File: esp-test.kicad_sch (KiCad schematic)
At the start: 77 parts, among them J1 AudioPlug3, J2 Micro_SD_Card_Det1, J3 USB_C_Receptacle_USB2.0_14P, J4 USB_C_Receptacle_USB2.0_14P, J5 Micro_SD_Card_Det2, SW1 Volume Up, SW2 Volume Down, SW3 Up, SW4 Down, SW5 Left, SW6 Right, SW7 SW_SPST, U1 ESP32-S3-WROOM-1, U2 AP2112K-3.3, U4 AP2112K-3.3

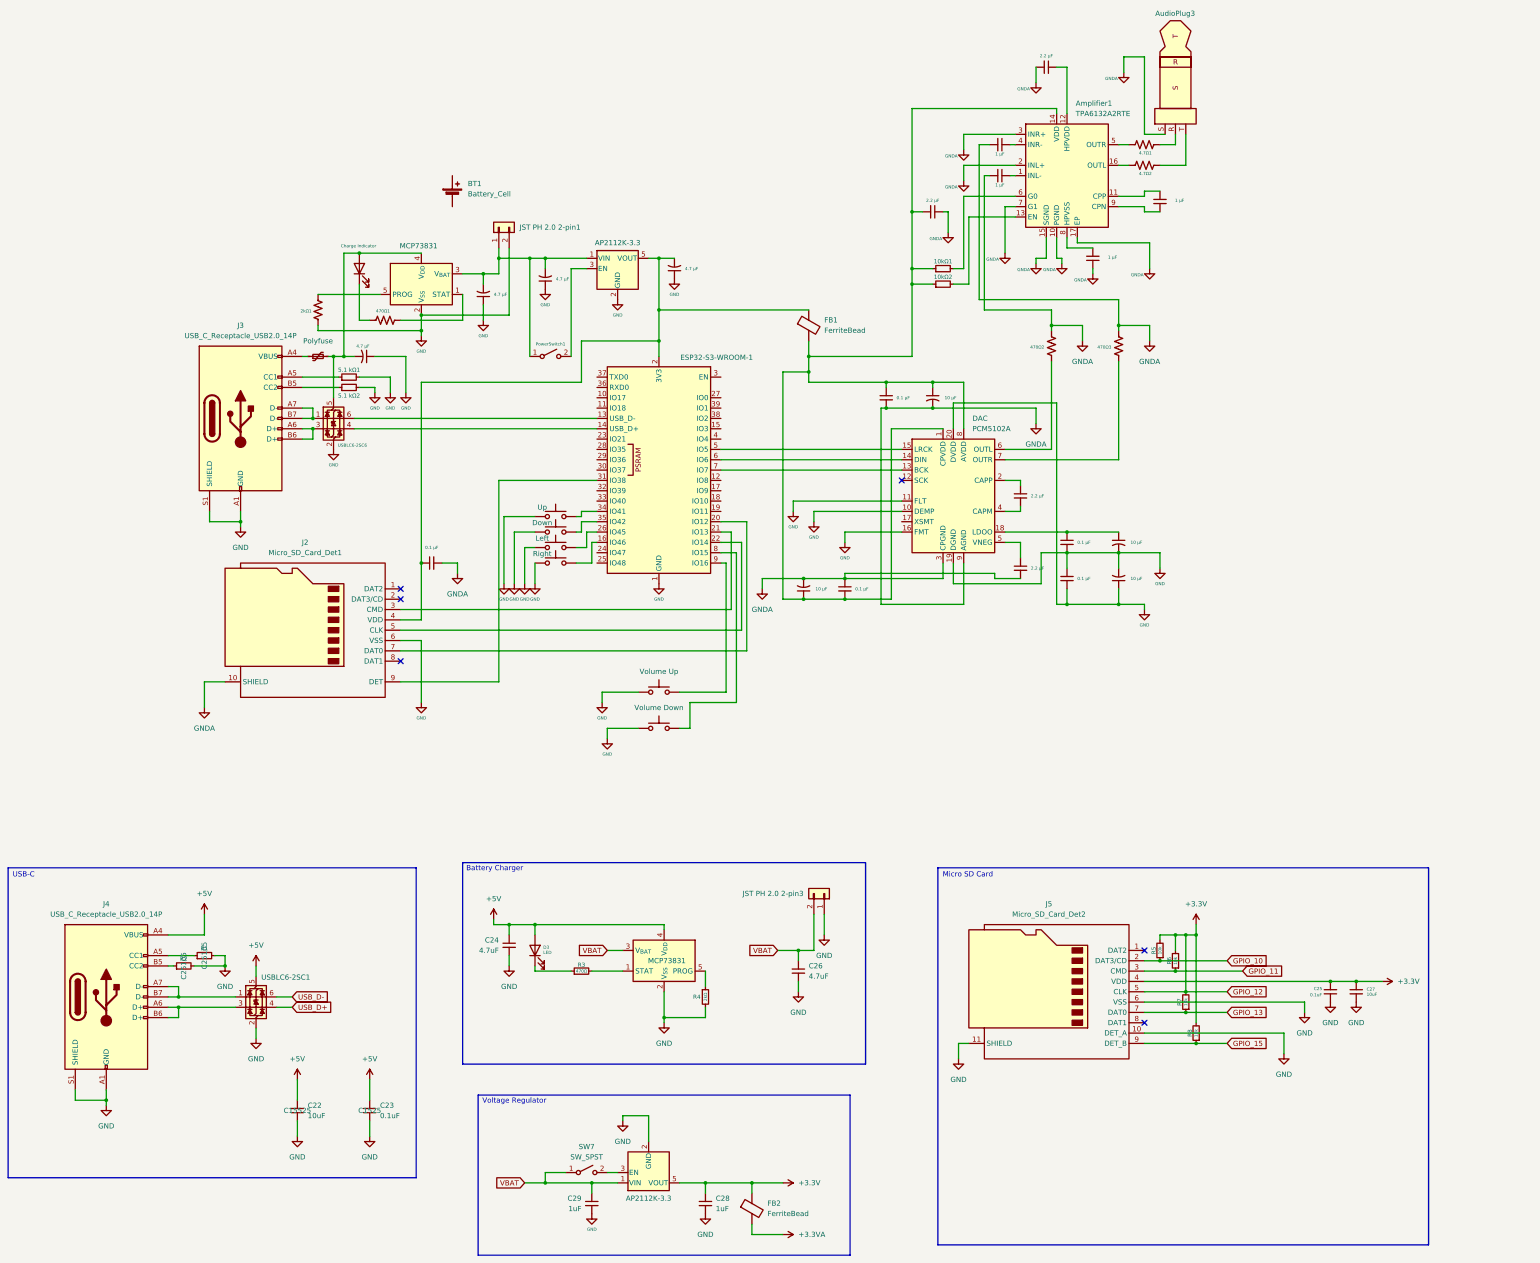
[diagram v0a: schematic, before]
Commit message: work
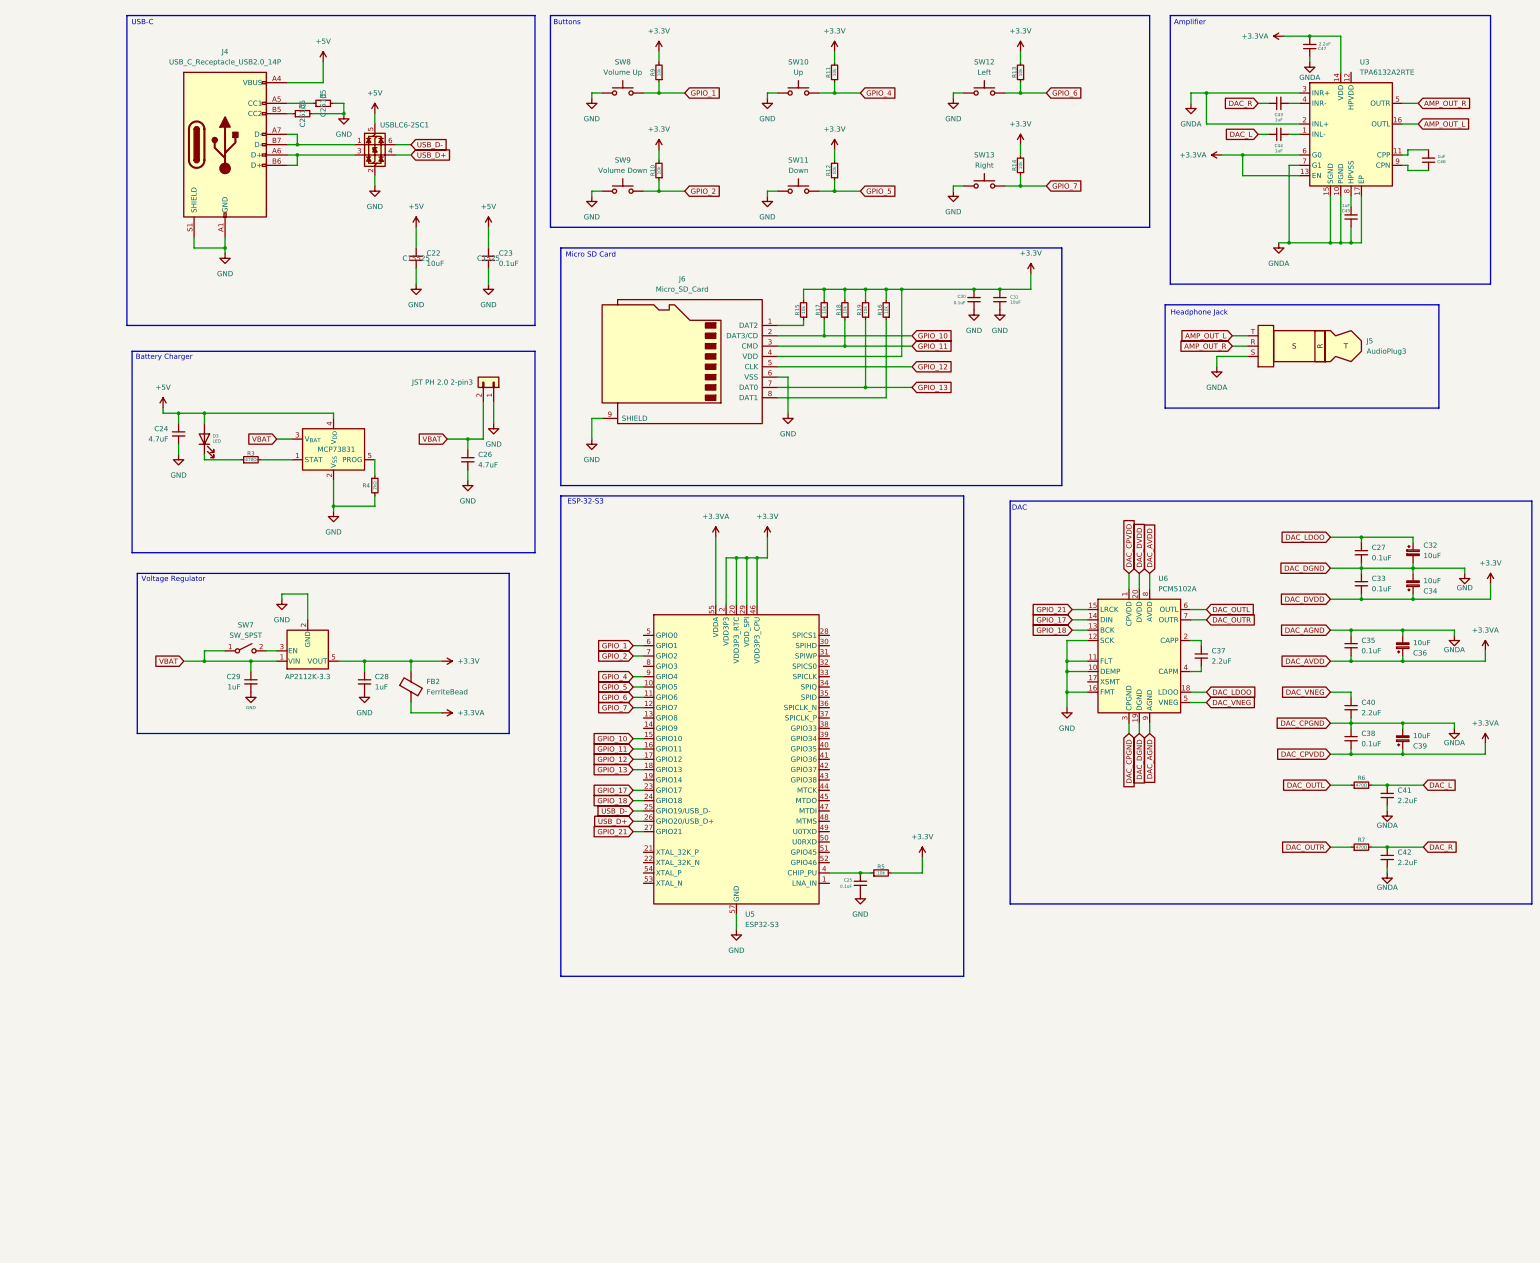
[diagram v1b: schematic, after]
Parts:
- removed 10kΩ1, 10kΩ2: R_Small, symbol Device:R_Small
- removed 2kΩ1, 4.7Ω1, 4.7Ω2, 470Ω1, 470Ω2, 470Ω3: R_US, symbol Device:R_US
- removed 5.1 kΩ1: R_Small, symbol Device:R_Small
- removed 5.1 kΩ2: R_Small, symbol Device:R_Small
- removed Amplifier1: TPA6132A2RTE, Package_DFN_QFN:WQFN-16-1EP_3x3mm_P0.5mm_EP1.6x1.6mm_ThermalVias, symbol Amplifier_Audio:TPA6132A2RTE
- removed BT1: Battery_Cell, symbol Device:Battery_Cell
- removed C1, C2, C3, C4: 4.7 µF, symbol Device:C_Small_US
- removed C10, C14, C21, C6, C8: 0.1 µF, symbol Device:C_Small
- removed C11, C13, C5, C9: 10 µF, symbol Device:C_Small_US
- removed C12, C17, C18, C7: 2.2 µF, symbol Device:C_Small
- removed C15, C16, C19, C20: 1 µF, symbol Device:C_Small
- removed D1: Charge Indicator, symbol Device:LED
- removed DAC: PCM5102A, Package_SO:TSSOP-20_4.4x6.5mm_P0.65mm, symbol Audio:PCM5102A
- removed F1: Polyfuse, symbol Device:Polyfuse_Small
- removed FB1: FerriteBead, symbol Device:FerriteBead
- removed J1: AudioPlug3, symbol Connector_Audio:AudioPlug3
- removed J2: Micro_SD_Card_Det1, symbol Connector:Micro_SD_Card_Det1
- removed J3: USB_C_Receptacle_USB2.0_14P, symbol Connector:USB_C_Receptacle_USB2.0_14P
- removed J5: Micro_SD_Card_Det2, Connector_Card:microSD_HC_Hirose_DM3AT-SF-PEJM5, symbol Connector:Micro_SD_Card_Det2
- removed JST PH 2.0 2-pin1: Conn_01x02, symbol Connector_Generic:Conn_01x02
- removed MCP73831: MCP73831-2-OT, Package_TO_SOT_SMD:SOT-23-5, symbol Battery_Management:MCP73831-2-OT
- removed PowerSwitch1: SW_SPST, symbol Switch:SW_SPST
- removed R8: 10k, symbol Device:R_Small
- removed SW1: Volume Up, symbol Switch:SW_Push
- removed SW2: Volume Down, symbol Switch:SW_Push
- removed SW3: Up, symbol Switch:SW_Push
- removed SW4: Down, symbol Switch:SW_Push
- removed SW5: Left, symbol Switch:SW_Push
- removed SW6: Right, symbol Switch:SW_Push
- removed U1: ESP32-S3-WROOM-1, RF_Module:ESP32-S3-WROOM-1, symbol RF_Module:ESP32-S3-WROOM-1
- removed U2: AP2112K-3.3, Package_TO_SOT_SMD:SOT-23-5, symbol Regulator_Linear:AP2112K-3.3
- removed USBLC6-2SC6: USBLC6-2SC6, Package_TO_SOT_SMD:SOT-23-6, symbol Power_Protection:USBLC6-2SC6
- added C30, C33, C35, C38: 0.1uF, symbol Device:C_Small
- added C31: 10uF, symbol Device:C_Small
- added C32, C34, C36, C39: 10uF, symbol Device:C_Polarized_Small
- added C37, C40, C41, C42, C47: 2.2uF, symbol Device:C_Small
- added C43, C44, C45, C46: 1uF, symbol Device:C_Small
- added J5: AudioPlug3, symbol Connector_Audio:AudioPlug3
- added J6: Micro_SD_Card, Connector_Card:microSD_HC_Molex_47219-2001, symbol Connector:Micro_SD_Card
- added R10, R11, R12, R13, R14, R15, R16, R17, R18, R19, R9: 10k, symbol Device:R_Small
- added SW10: Up, symbol Switch:SW_Push
- added SW11: Down, symbol Switch:SW_Push
- added SW12: Left, symbol Switch:SW_Push
- added SW13: Right, symbol Switch:SW_Push
- added SW8: Volume Up, symbol Switch:SW_Push
- added SW9: Volume Down, symbol Switch:SW_Push
- added U3: TPA6132A2RTE, Package_DFN_QFN:WQFN-16-1EP_3x3mm_P0.5mm_EP1.6x1.6mm_ThermalVias, symbol Amplifier_Audio:TPA6132A2RTE
- added U5: ESP32-S3, Package_DFN_QFN:QFN-56-1EP_7x7mm_P0.4mm_EP4x4mm, symbol MCU_Espressif:ESP32-S3
- added U6: PCM5102A, Package_SO:TSSOP-20_4.4x6.5mm_P0.65mm, symbol Audio:PCM5102A
- C27: value 10uF -> 0.1uF
- R6, R7: value 10k -> 470Ω
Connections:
- net +3.3V: now also C30.2, C31.1, C33.2, C34.1, J6.4 (VDD), R10.2, R11.2, R12.2, R13.2, R14.2, R15.2, R16.2, R17.2, R18.2, R19.2, R9.2, U5.2 (VDD3P3), U5.20 (VDD3P3_RTC), U5.29 (VDD_SPI), U5.3 (VDD3P3), U5.46 (VDD3P3_CPU), U6.20 (DVDD); no longer C25.2, C27.1, R6.2, R7.2
- net +3.3VA: now also C35.2, C36.1, C38.2, C39.1, C47.2, U3.13 (EN), U3.14 (VDD), U3.6 (G0), U5.55 (VDDA), U5.56 (VDDA), U6.1 (CPVDD), U6.8 (AVDD)
- net GND: now also C30.1, C31.2, C32.2, C33.1, C34.2, J6.6 (VSS), J6.9 (SHIELD), SW10.1, SW11.1, SW12.1, SW13.1, SW8.1, SW9.1, U5.57 (GND), U6.10 (DEMP), U6.11 (FLT), U6.12 (SCK), U6.16 (FMT), U6.19 (DGND)
- net GNDA: now also C35.1, C36.2, C38.1, C39.2, C40.2, C41.2, C42.2, C45.1, C47.1, J5.S, U3.10 (PGND), U3.15 (SGND), U3.17 (EP), U3.2 (INL+), U3.3 (INR+), U3.7 (G1), U6.3 (CPGND), U6.9 (AGND)
- net GPIO_10: now also J6.2 (DAT3/CD), R17.1, U5.15 (GPIO10); no longer R5.1
- net GPIO_11: now also J6.3 (CMD), R18.1, U5.16 (GPIO11); no longer R6.1
- net GPIO_13: now also J6.7 (DAT0), R19.1, U5.18 (GPIO13); no longer R7.1
- net USB_D+: now also U5.26 (GPIO20/USB_D+)
- net USB_D-: now also U5.25 (GPIO19/USB_D-)
- new net: C44.2, U3.1 (INL-)
- new net: C46.2, U3.11 (CPP)
- new net: C43.2, U3.4 (INR-)
- new net: C45.2, U3.8 (HPVSS)
- new net: C46.1, U3.9 (CPN)
- new net: J6.1 (DAT2), R15.1
- new net: C25.2, R5.1, U5.4 (CHIP_PU)
- new net: J6.8 (DAT1), R16.1
- new net: C37.1, U6.2 (CAPP)
- new net: C37.2, U6.4 (CAPM)
- new net AMP_OUT_L: J5.T, U3.16 (OUTL)
- new net AMP_OUT_R: J5.R, U3.5 (OUTR)
- new net DAC_L: C41.1, C44.1, R6.2
- new net DAC_LDOO: C27.1, C32.1, U6.18 (LDOO)
- new net DAC_OUTL: R6.1, U6.6 (OUTL)
- new net DAC_OUTR: R7.1, U6.7 (OUTR)
- new net DAC_R: C42.1, C43.1, R7.2
- new net DAC_VNEG: C40.1, U6.5 (VNEG)
- new net GPIO_1: R9.1, SW8.2, U5.6 (GPIO1)
- new net GPIO_12: J6.5 (CLK), U5.17 (GPIO12)
- new net GPIO_17: U5.23 (GPIO17), U6.14 (DIN)
- new net GPIO_18: U5.24 (GPIO18), U6.13 (BCK)
- new net GPIO_2: R10.1, SW9.2, U5.7 (GPIO2)
- new net GPIO_21: U5.27 (GPIO21), U6.15 (LRCK)
- new net GPIO_4: R11.1, SW10.2, U5.9 (GPIO4)
- new net GPIO_5: R12.1, SW11.2, U5.10 (GPIO5)
- new net GPIO_6: R13.1, SW12.2, U5.11 (GPIO6)
- new net GPIO_7: R14.1, SW13.2, U5.12 (GPIO7)
- no-connect marks 6 -> 0
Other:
- note added: "Amplifier"
- note added: "Buttons"
- note added: "DAC"
- note added: "ESP-32-S3"
- note added: "Headphone Jack"
- moved on the sheet: C22, C23, C24, C26, C28, C29, D3, FB2, J4, JST PH 2.0 2-pin3, MCP73831, R1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
